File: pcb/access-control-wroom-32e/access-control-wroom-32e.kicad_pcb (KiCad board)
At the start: 2 copper layers, 71.4 x 63.3 mm, 39 parts, among them J1 CON_I2C, K1 G5LE-1, U1 ESP32-DevKitC

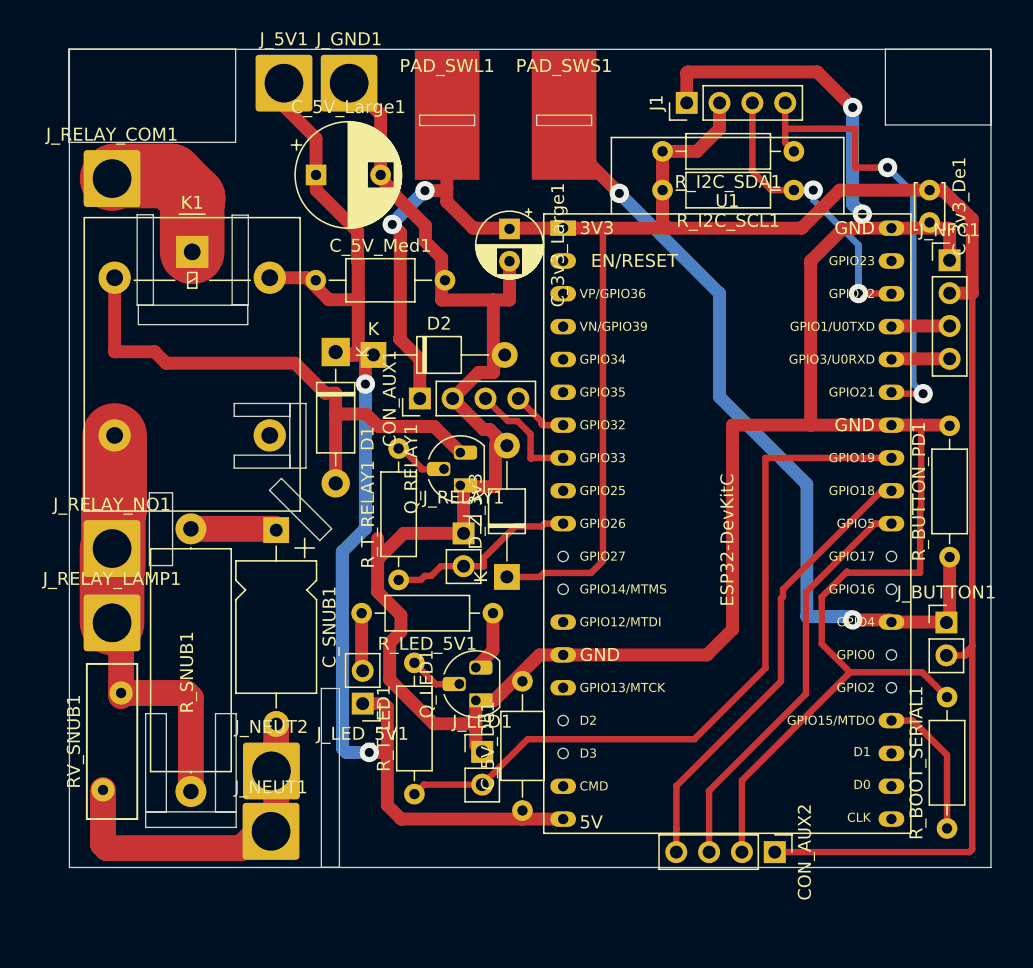
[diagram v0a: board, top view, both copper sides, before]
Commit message: Further optimisation
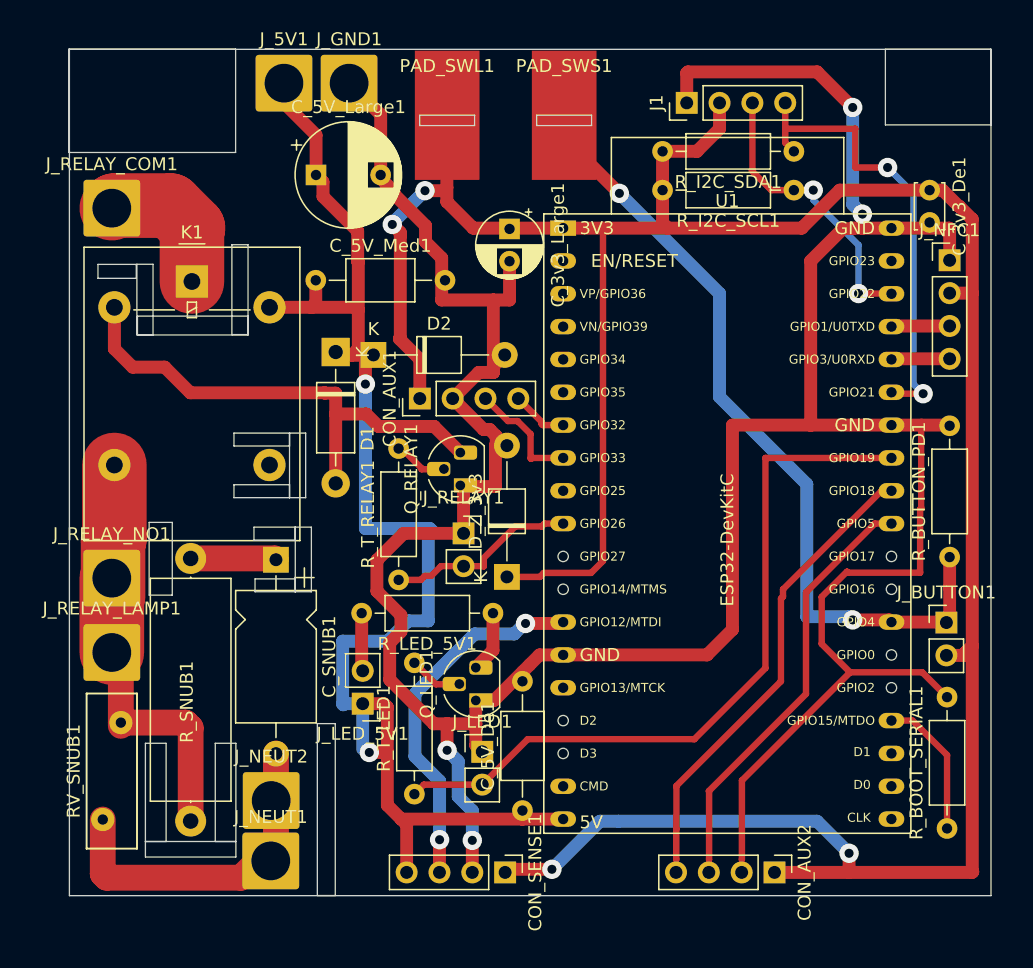
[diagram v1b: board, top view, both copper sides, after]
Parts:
- added CON_SENSE1: Conn_01x04_Socket, Connector_PinHeader_2.54mm:PinHeader_1x04_P2.54mm_Vertical, F.Cu at (33.1, 63.7)
- moved RV_SNUB1 2.29 mm to (3.38, 52.1)
- moved C_SNUB1 2.29 mm to (15.4, 39.5)
- moved J_NEUT1 2.29 mm to (15.0, 62.8)
- moved J_NEUT2 2.29 mm to (15.0, 58.1)
- moved J_RELAY_COM1 2.29 mm to (2.68, 12.3)
- moved J_RELAY_LAMP1 2.29 mm to (2.68, 46.7)
- moved J_RELAY_NO1 2.29 mm to (2.68, 40.9)
- moved K1 2.29 mm to (8.88, 18.0)
- moved R_SNUB1 2.29 mm to (8.78, 59.7)
- moved CON_AUX2 1.57 mm to (54.0, 63.7)
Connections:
- U1 pad : Net-(CON_AUX2-Pin_3) -> (no net)
- U1 pad 13: unconnected-(U1-MTDI/GPIO12/ADC2_CH5-Pad13) -> Net-(CON_SENSE1-Pin_3)
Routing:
- net +3V3: track 185.0 -> 217.5 mm, vias 2 -> 4
- net Net-(CON_SENSE1-Pin_3): track 0.00 -> 28.6 mm, vias 0 -> 2
- net +5V: track 92.1 -> 107.9 mm
- net GND: track 247.5 -> 258.7 mm, vias 2 -> 4
- net Net-(D1-A): track 42.0 -> 39.6 mm
- net Net-(CON_AUX2-Pin_3): track 32.0 -> 32.6 mm
- net Net-(CON_AUX2-Pin_4): track 35.3 -> 35.9 mm
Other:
- board size 71.4 x 63.3 mm -> 71.4 x 65.5 mm
